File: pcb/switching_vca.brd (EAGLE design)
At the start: 100 x 22 mm, 37 parts, among them Q101 PMOS, Q102 NJFET, U101 LM319, U102 LF353D, U103 LF353D, U701 V_REG_LDOSMD

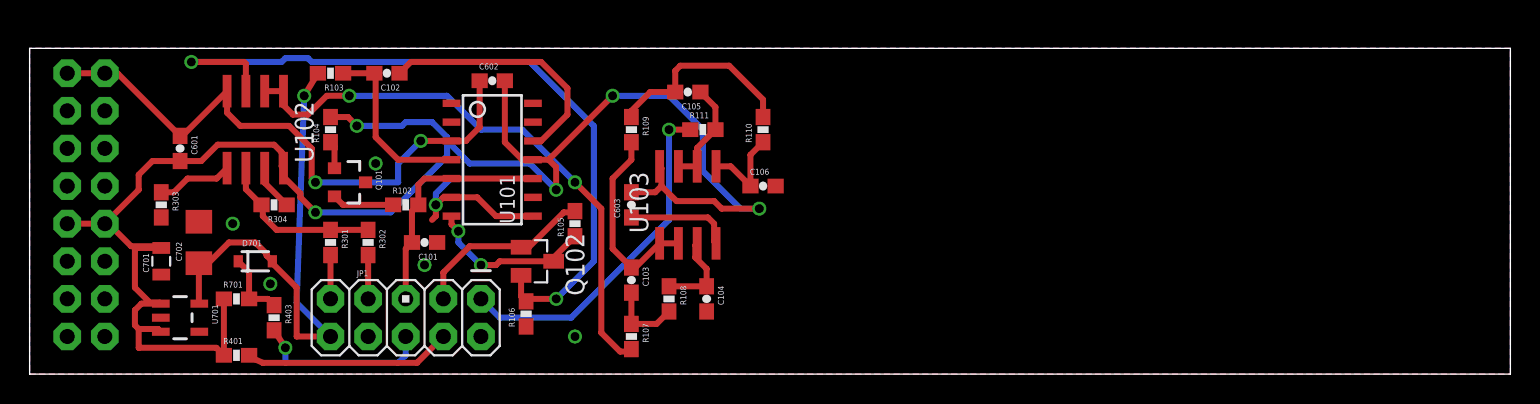
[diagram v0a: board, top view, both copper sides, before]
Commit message: Routed the board with a travesty of VIAs
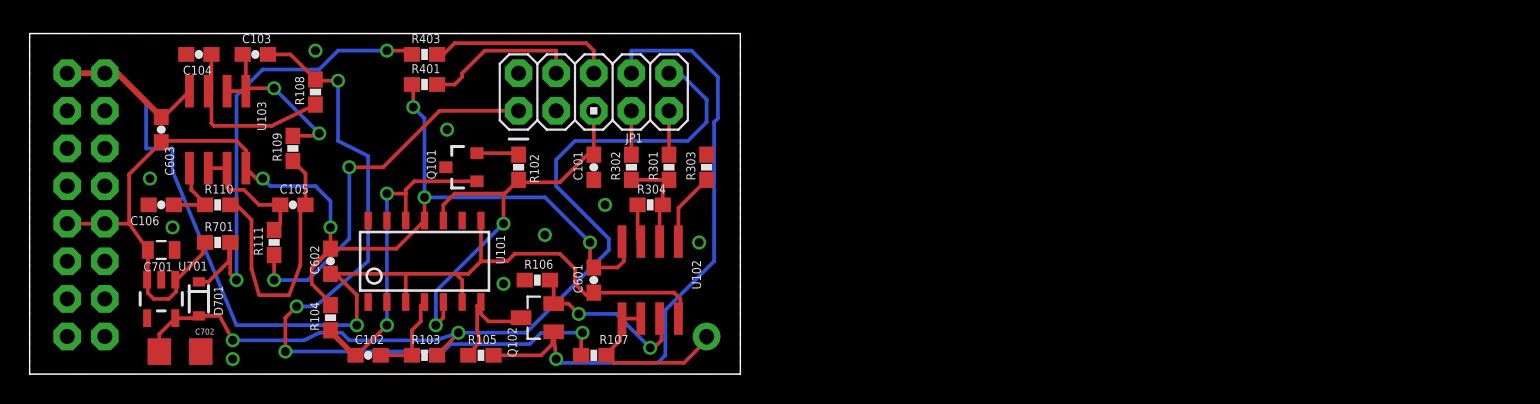
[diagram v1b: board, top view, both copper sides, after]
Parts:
- added TP101: (no value), SparkFun:1X01
- added U$1: (no value), SparkFun:OSHW-LOGO-L
- moved C106 40.7 mm to (8.89, 11.4), turned to 180 degrees
- moved C104 38.1 mm to (11.4, 21.6), turned to 180 degrees
- moved R110 37.2 mm to (12.7, 11.4), turned to 0 degrees
- moved R303 36.9 mm to (45.7, 14.0), turned to 90 degrees
- moved U103 32.2 mm to (12.7, 16.5), turned to 180 degrees
- moved C603 32.2 mm to (8.89, 16.5), turned to 270 degrees
- moved R111 29.9 mm to (16.5, 8.89), turned to 90 degrees
- moved C103 29.6 mm to (15.2, 21.6), turned to 0 degrees
- moved C601 29.3 mm to (38.1, 6.35), turned to 90 degrees
- moved U102 28.5 mm to (41.9, 6.35), turned to 0 degrees
- moved C105 27.7 mm to (17.8, 11.4), turned to 0 degrees
- moved R108 27.7 mm to (19.3, 19.1), turned to 90 degrees
- moved R304 25.4 mm to (41.9, 11.4), turned to 0 degrees
- moved R301 23.4 mm to (43.2, 14.0), turned to 90 degrees
- moved R109 22.9 mm to (17.8, 15.2), turned to 90 degrees
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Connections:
- net IN: now also JP1.8; no longer JP1.3
- net N$15: now also TP101.1
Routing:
- net N$7: track 5.00 -> 50.4 mm, vias 0 -> 4
- net N$6: track 51.5 -> 11.9 mm
- net +12V: track 120.1 -> 80.6 mm
- net IN: track 12.4 -> 43.1 mm, vias 0 -> 1
- net 5V3: track 4.71 -> 32.3 mm, vias 0 -> 2
- net N$15: track 38.6 -> 12.1 mm, vias 2 -> 1
- net +5V: track 35.9 -> 61.4 mm, vias 1 -> 2
- net -12V: track 58.6 -> 78.3 mm, vias 3 -> 1
- net INT: track 16.0 -> 28.3 mm, vias 0 -> 2
- net N$8: track 5.81 -> 12.4 mm
- net N$4: track 12.2 -> 6.06 mm
- net N$: track 19.1 -> 24.9 mm, vias 0 -> 2
- net N$11: track 13.5 -> 18.7 mm
- net R301: track 11.2 -> 6.97 mm
- net N$3: track 11.4 -> 7.83 mm, vias 2 -> 0
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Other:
- board size 100 x 22 mm -> 48 x 23 mm
- board text added: "Digitally Controlled Amplifier Alpha"
